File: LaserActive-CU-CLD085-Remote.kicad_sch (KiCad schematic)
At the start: 35 parts, among them IC1 D6600CS, K0 Button, K1 Button, K10 Button, K11 Button, K12 Button, K16 Button, K18 Button, K19 Button, K2 Button, K20 Button, K24 Button, K25 Button, K26 Button, K27 Button, K28 Button, K29 Button, K3 Button, K32 Button, K33 Button, K34 Button, K35 Button, K36 Button, K4 Button, K7 Button, Q1 NPN, X1 Crystal

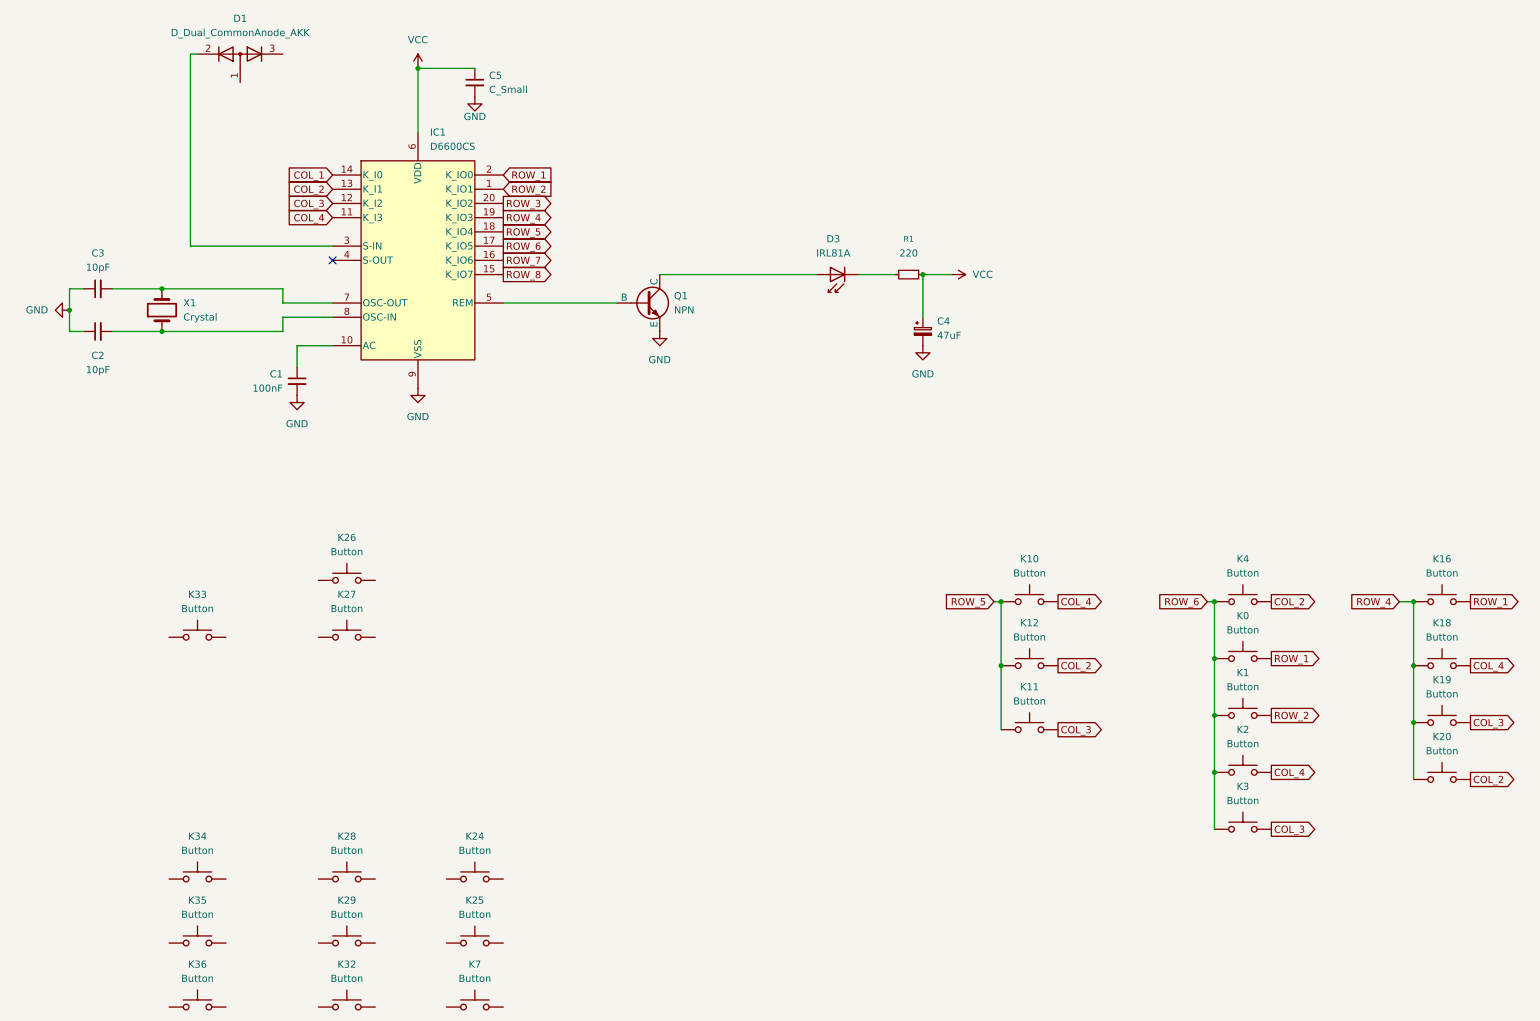
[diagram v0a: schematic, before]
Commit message: Update Schematics and PCB
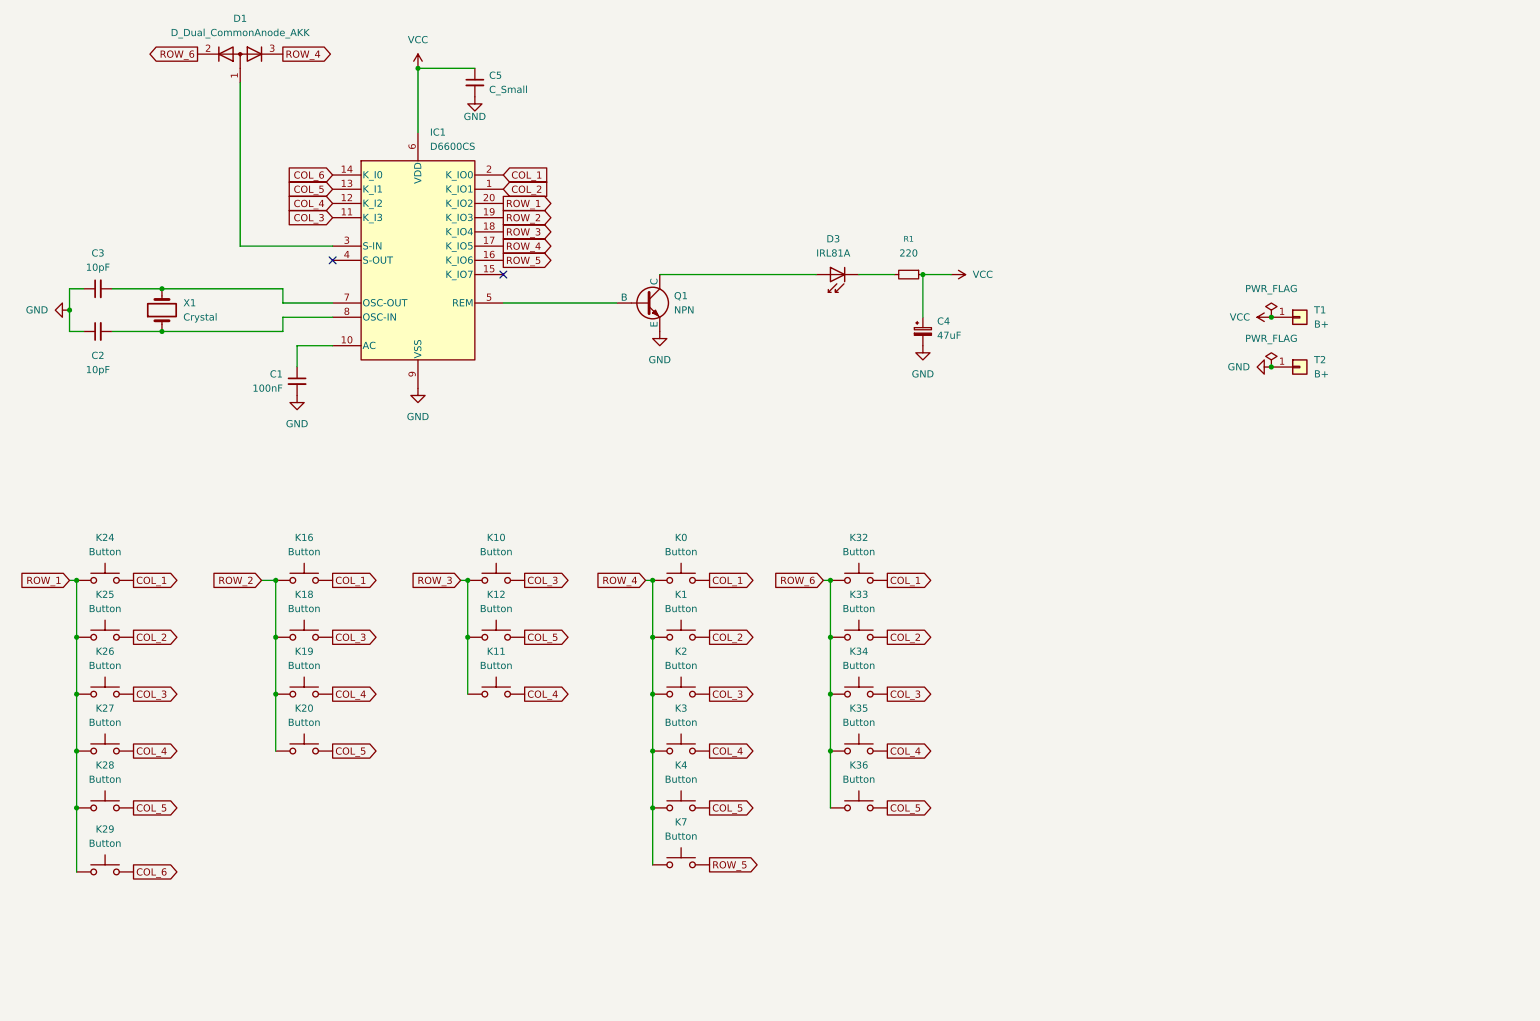
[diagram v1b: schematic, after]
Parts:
- added T1, T2: B+, Connector_PinHeader_2.54mm:PinHeader_1x01_P2.54mm_Vertical, symbol Connector_Generic:Conn_01x01
- C4: footprint Capacitor_THT:CP_Radial_D5.0mm_P2.00mm -> Pioneer:Electrolytic_P2.50mm
- IC1: footprint Package_DIP:DIP-20_W7.62mm_Socket_LongPads -> Pioneer:DIP-20_W7.62mm_P1.76mm
- K0, K1, K10, K11, K12, K16, K18, K19, K2, K20, K24, K25, K26, K27, K28, K29, K3, K32, K33, K34, K35, K36, K4, K7: footprint Button_Switch_SMD:SW_SPST_CK_KXT3 -> Pioneer:Button
- Q1: footprint Package_TO_SOT_THT:TO-220-3_Vertical -> Pioneer:TO-220-3
- X1: footprint Crystal:Crystal_HC18-U_Vertical -> Pioneer:Crystal
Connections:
- net ROW_7 is gone; now on net ROW_5: IC1.16 (K_IO6)
- net COL_1: now also IC1.2 (K_IO0), K0.2, K16.2, K24.2, K32.2; no longer IC1.14 (K_I0)
- net COL_2: now also IC1.1 (K_IO1), K1.1, K25.2, K33.1; no longer IC1.13 (K_I1), K12.2, K20.2, K4.2
- net COL_3: now also IC1.11 (K_I3), K10.2, K18.2, K2.1, K26.2, K34.2; no longer IC1.12 (K_I2), K11.1, K19.2, K3.1
- net COL_4: now also IC1.12 (K_I2), K11.1, K19.2, K27.1, K3.1, K35.2; no longer IC1.11 (K_I3), K10.2, K18.2, K2.1
- net GND: now also T2.1 (Pin_1)
- net ROW_1: now also IC1.20 (K_IO2), K24.1, K25.1, K26.1, K27.2, K28.1, K29.2; no longer IC1.2 (K_IO0), K0.2, K16.2
- net ROW_2: now also IC1.19 (K_IO3), K16.1, K18.1, K19.1, K20.1; no longer IC1.1 (K_IO1), K1.1
- net ROW_3: now also IC1.18 (K_IO4), K10.1, K11.2, K12.1; no longer IC1.20 (K_IO2)
- net ROW_4: now also D1.3 (K), IC1.17 (K_IO5), K0.1, K1.2, K2.2, K3.2, K4.1, K7.2; no longer IC1.19 (K_IO3), K16.1, K18.1, K19.1, K20.1
- net ROW_5: now also K7.1; no longer IC1.18 (K_IO4), K10.1, K11.2, K12.1
- net ROW_6: now also D1.2 (K), K32.1, K33.2, K34.1, K35.1, K36.2; no longer IC1.17 (K_IO5), K0.1, K1.2, K2.2, K3.2, K4.1
- net VCC: now also T1.1 (Pin_1)
- net at IC1.3 (S-IN): now also D1.1 (A); no longer D1.2 (K)
- net COL_5: now reaches K28.2
- net COL_5: now also IC1.13 (K_I1), K12.2, K20.2, K36.1, K4.2
- net COL_6: now reaches K29.1
- net COL_6: now also IC1.14 (K_I0)
- net ROW_8: no longer names the net of IC1.15 (K_IO7)
- no-connect marks 1 -> 2
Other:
- moved on the sheet: K0, K1, K10, K11, K12, K16, K18, K19, K2, K20, K24, K25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

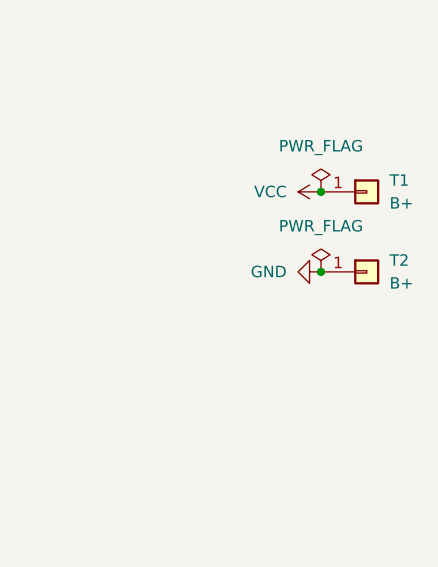
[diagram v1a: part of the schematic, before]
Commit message: fix extra b+
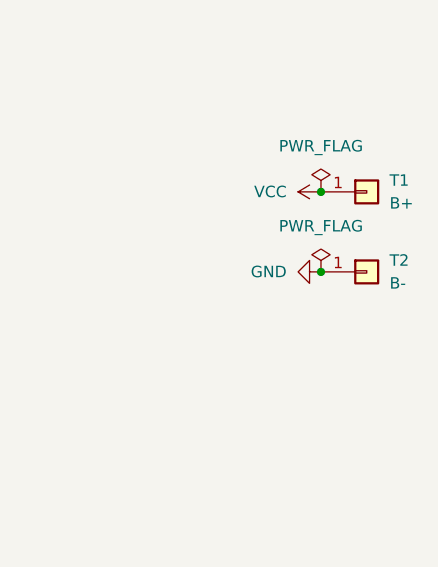
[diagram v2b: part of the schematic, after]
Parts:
- T2: value B+ -> B-
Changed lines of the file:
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@@
 			)
 		)
-		(property "Value" "B+"
+		(property "Value" "B-"
 			(at 245.11 80.0099 0)
 			(effects

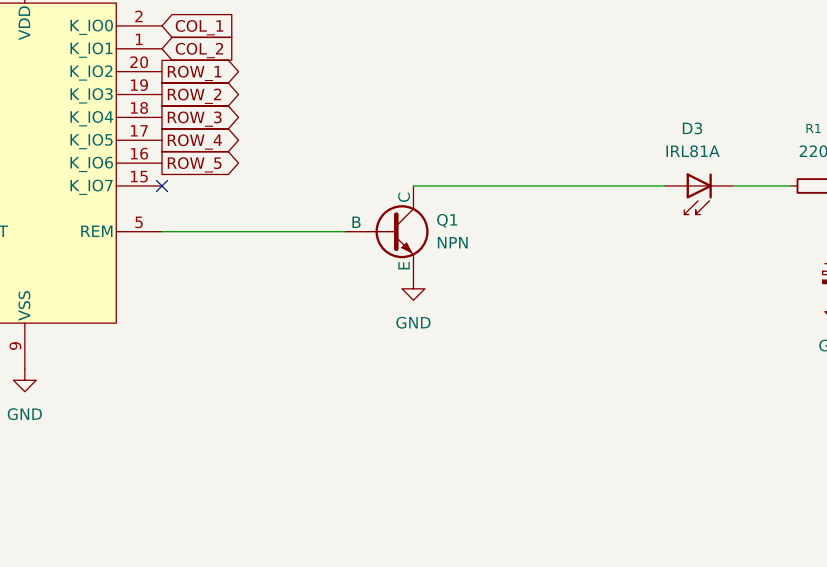
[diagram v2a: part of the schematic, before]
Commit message: Updates
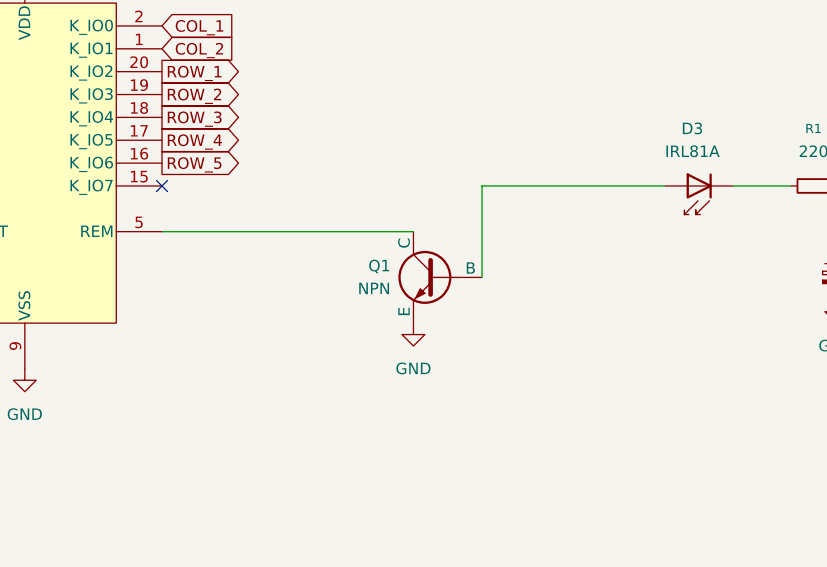
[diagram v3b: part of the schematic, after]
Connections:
- net at IC1.5 (REM): now also Q1.1 (C); no longer Q1.2 (B)
- net at D3.2 (A): now also Q1.2 (B); no longer Q1.1 (C)
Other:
- moved on the sheet: Q1
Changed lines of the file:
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@@
 	(wire
 		(pts
-			(xy 100.33 67.31) (xy 120.65 67.31)
+			(xy 100.33 67.31) (xy 128.27 67.31)
 		)
 		(stroke
@@
 	(wire
 		(pts
-			(xy 128.27 62.23) (xy 156.21 62.23)
-		)
-		(stroke
-			(width 0)
-			(type default)
-		)
-	)
-	(wire
-		(pts
 			(xy 69.85 57.15) (xy 53.34 57.15)
 		)
@@
 	(wire
 		(pts
+			(xy 135.89 62.23) (xy 156.21 62.23)
+		)
+		(stroke
+			(width 0)
+			(type default)
+		)
+	)
+	(wire
+		(pts
 			(xy 22.86 72.39) (xy 25.4 72.39)
 		)
@@
 		(pts
 			(xy 30.48 64.77) (xy 39.37 64.77)
+		)
+		(stroke
+			(width 0)
+			(type default)
+		)
+	)
+	(wire
+		(pts
+			(xy 135.89 62.23) (xy 135.89 72.39)
 		)
 		(stroke
@@
 	(symbol
 		(lib_id "power:GND")
-		(at 128.27 72.39 0)
+		(at 128.27 77.47 0)
 		(unit 1)
 		(exclude_from_sim no)
@@
 		(fields_autoplaced yes)
 		(property "Reference" "#PWR04"
-			(at 128.27 78.74 0)
+			(at 128.27 83.82 0)
 			(effects
 				(font
@@
 		)
 		(property "Value" "GND"
+			(at 128.27 82.55 0)
+			(effects
+				(font
+					(size 1.27 1.27)
+				)
+			)
+		)
+		(property "Footprint" ""
 			(at 128.27 77.47 0)
 			(effects
@@
 					(size 1.27 1.27)
 				)
-			)
-		)
-		(property "Footprint" ""
-			(at 128.27 72.39 0)
-			(effects
-				(font
-					(size 1.27 1.27)
-				)
 				(hide yes)
 			)
 		)
 		(property "Datasheet" ""
-			(at 128.27 72.39 0)
+			(at 128.27 77.47 0)
 			(effects
 				(font
@@
 		)
 		(property "Description" "Power symbol creates a global label with name \"GND\" , ground"
-			(at 128.27 72.39 0)
+			(at 128.27 77.47 0)
 			(effects
 				(font
@@
 	(symbol
 		(lib_id "Simulation_SPICE:NPN")
-		(at 125.73 67.31 0)
+		(at 130.81 72.39 0)
+		(mirror y)
 		(unit 1)
 		(exclude_from_sim no)
@@
 		(on_board yes)
 		(dnp no)
-		(fields_autoplaced yes)
 		(property "Reference" "Q1"
-			(at 130.81 66.0399 0)
+			(at 125.73 71.1199 0)
 			(effects
 				(font
@@
 		)
 		(property "Value" "NPN"
-			(at 130.81 68.5799 0)
+			(at 125.73 73.6599 0)
 			(effects
 				(font
@@
 		)
 		(property "Footprint" "Pioneer:TO-220-3"
-			(at 189.23 67.31 0)
+			(at 67.31 72.39 0)
 			(effects
 				(font
@@
 		)
 		(property "Datasheet" ""
-			(at 189.23 67.31 0)
+			(at 67.31 72.39 0)
 			(effects
 				(font
@@
 		)
 		(property "Description" ""
-			(at 125.73 67.31 0)
+			(at 130.81 72.39 0)
 			(effects
 				(font
@@
 		)
 		(property "Sim.Device" "NPN"
-			(at 125.73 67.31 0)
+			(at 130.81 72.39 0)
 			(effects
 				(font
@@
 		)
 		(property "Sim.Type" "GUMMELPOON"
-			(at 125.73 67.31 0)
+			(at 130.81 72.39 0)
 			(effects
 				(font
@@
 		)
 		(property "Sim.Pins" "1=C 2=B 3=E"
-			(at 125.73 67.31 0)
-			(effects
-				(font
+			(at 130.81 72.39 0)
+			(effects
+				(font
